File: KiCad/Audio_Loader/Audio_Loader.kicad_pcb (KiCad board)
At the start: 2 copper layers, 58.4 x 35.6 mm, 22 parts, among them J1 USB_B_Micro, J2 DB9_Female_MountingHoles, J3 AudioJack2, Q1 BC547, U1 LM741, U2 LM393, U3 MAX202

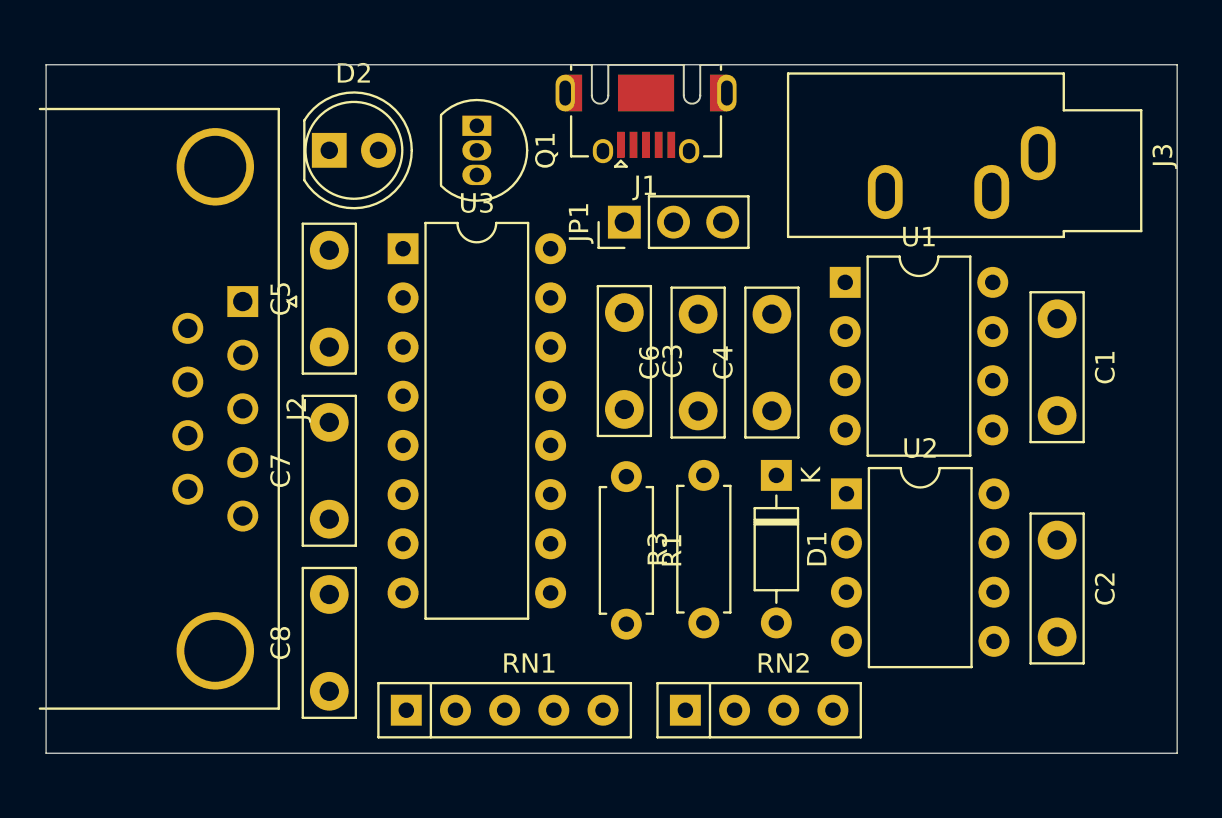
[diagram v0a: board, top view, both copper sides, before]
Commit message: Audio Loader PCB Rev. 0
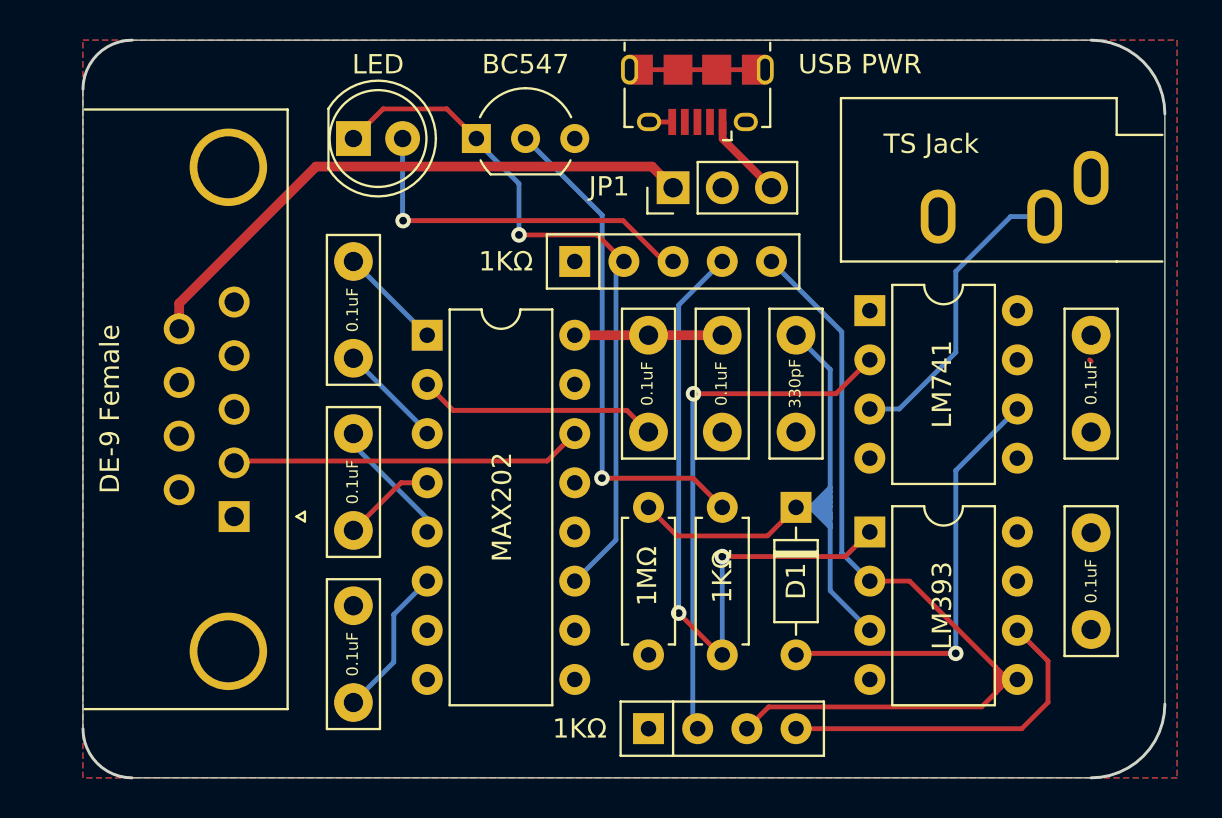
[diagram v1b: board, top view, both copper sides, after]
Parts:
- J1: value USB_B_Micro -> USB PWR; footprint Connector_USB:USB_Micro-AB_Molex_47590-0001 -> Connector_USB:USB_Micro-B_Amphenol_10118194_Horizontal
- J2: value DB9_Female_MountingHoles -> DE-9 Female; footprint Connector_Dsub:DSUB-9_Male_Horizontal_P2.77x2.84mm_EdgePinOffset7.70mm_Housed_MountingHolesOffset9.12mm -> Connector_Dsub:DSUB-9_Female_Horizontal_P2.77x2.84mm_EdgePinOffset4.94mm_Housed_MountingHolesOffset7.48mm
- J3: value AudioJack2 -> TS Jack
- Q1: footprint Package_TO_SOT_THT:TO-92_Inline -> Package_TO_SOT_THT:TO-92_Inline_Wide
- RN1: value R_Network04 -> 1KΩ
- RN2: value R_Network03 -> 1KΩ
- moved RN1 24.8 mm to (136.4, 85.8)
- moved J2 11.1 mm to (118.8, 98.9)
- moved C3 5.19 mm to (144.0, 89.6)
- moved C6 4.68 mm to (140.2, 89.6), turned to 270 degrees
- moved U3 4.64 mm to (128.8, 89.6)
- moved JP1 3.08 mm to (141.5, 81.9)
- moved J3 3.01 mm to (163.0, 81.4)
- moved J1 2.65 mm to (142.7, 77.1)
- moved U2 2.31 mm to (151.6, 99.7)
- moved RN2 2.13 mm to (140.2, 109.9)
- moved R1 1.96 mm to (140.2, 98.5)
- moved C1 1.95 mm to (163.0, 89.6)
- moved D1 1.94 mm to (147.8, 98.5)
- moved U1 1.94 mm to (151.6, 88.3)
- moved R3 1.91 mm to (144.0, 106.1)
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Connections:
- RN1 pad 2: RN1a -> RN1c
- RN1 pad 3: RN1b -> RN1d
- RN1 pad 4: RN1c -> RN1b
- RN1 pad 5: RN1d -> RN1a
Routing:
- net RN1a: track 0.00 -> 48.5 mm
- net Net-(C4-Pad2): track 0.00 -> 39.8 mm
- net RN1c: track 0.00 -> 36.7 mm, vias 0 -> 1
- net RN1b: track 0.00 -> 35.5 mm, vias 0 -> 2
- net PIN_9: track 0.00 -> 30.0 mm
- net RN2a: track 0.00 -> 27.3 mm, vias 0 -> 1
- net Net-(Q1-Pad2): track 0.00 -> 26.0 mm, vias 0 -> 1
- net Net-(D1-Pad2): track 0.00 -> 22.3 mm, vias 0 -> 1
- net RN1d: track 0.00 -> 18.7 mm, vias 0 -> 1
- net Net-(J2-Pad2): track 0.00 -> 18.4 mm
- net RN2c: track 0.00 -> 18.0 mm
- net Net-(J3-PadT): track 0.00 -> 15.6 mm
- net Net-(C6-Pad2): track 0.00 -> 12.4 mm
- net Net-(C8-Pad1): track 0.00 -> 7.85 mm
- net VCC: track 0.00 -> 7.73 mm
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- added copper zone on B.Cu, net GND
- added copper zone on F.Cu, net VCC
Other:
- board size 58.4 x 35.6 mm -> 55.9 x 38.1 mm
- net class Power added: clearance 0.4, trace_width 0.5, via_dia 0.8, via_drill 0.4
- board text added: "MAX202"
- board text added: "ZF Audio Loader @tangent3D 2021 Rev. 0"
